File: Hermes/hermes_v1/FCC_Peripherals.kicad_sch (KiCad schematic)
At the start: 26 parts, among them J2 Connector_USB_B_Micro, J3 Conn_01x07, J4 Conn_02x07_Odd_Even, J5 Additional IO, J6 Micro_SD_Card, J7 IO Power, U5 MPU-6050, U6 MPL3115A2, U7 USBLC6-2P6

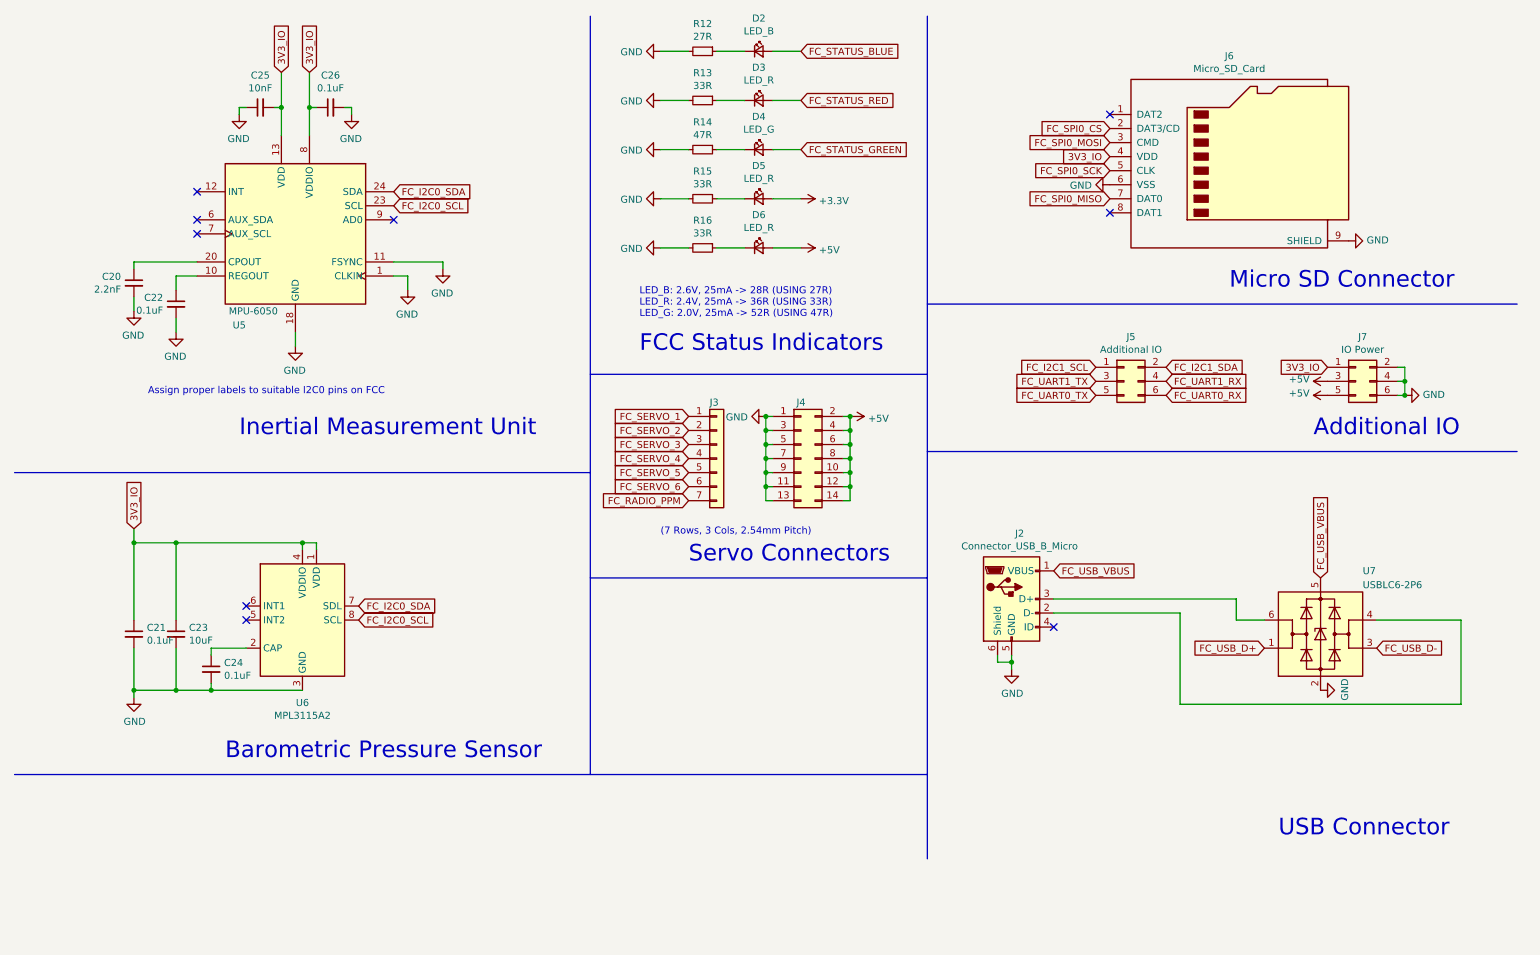
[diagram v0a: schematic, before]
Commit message: Hermes v2
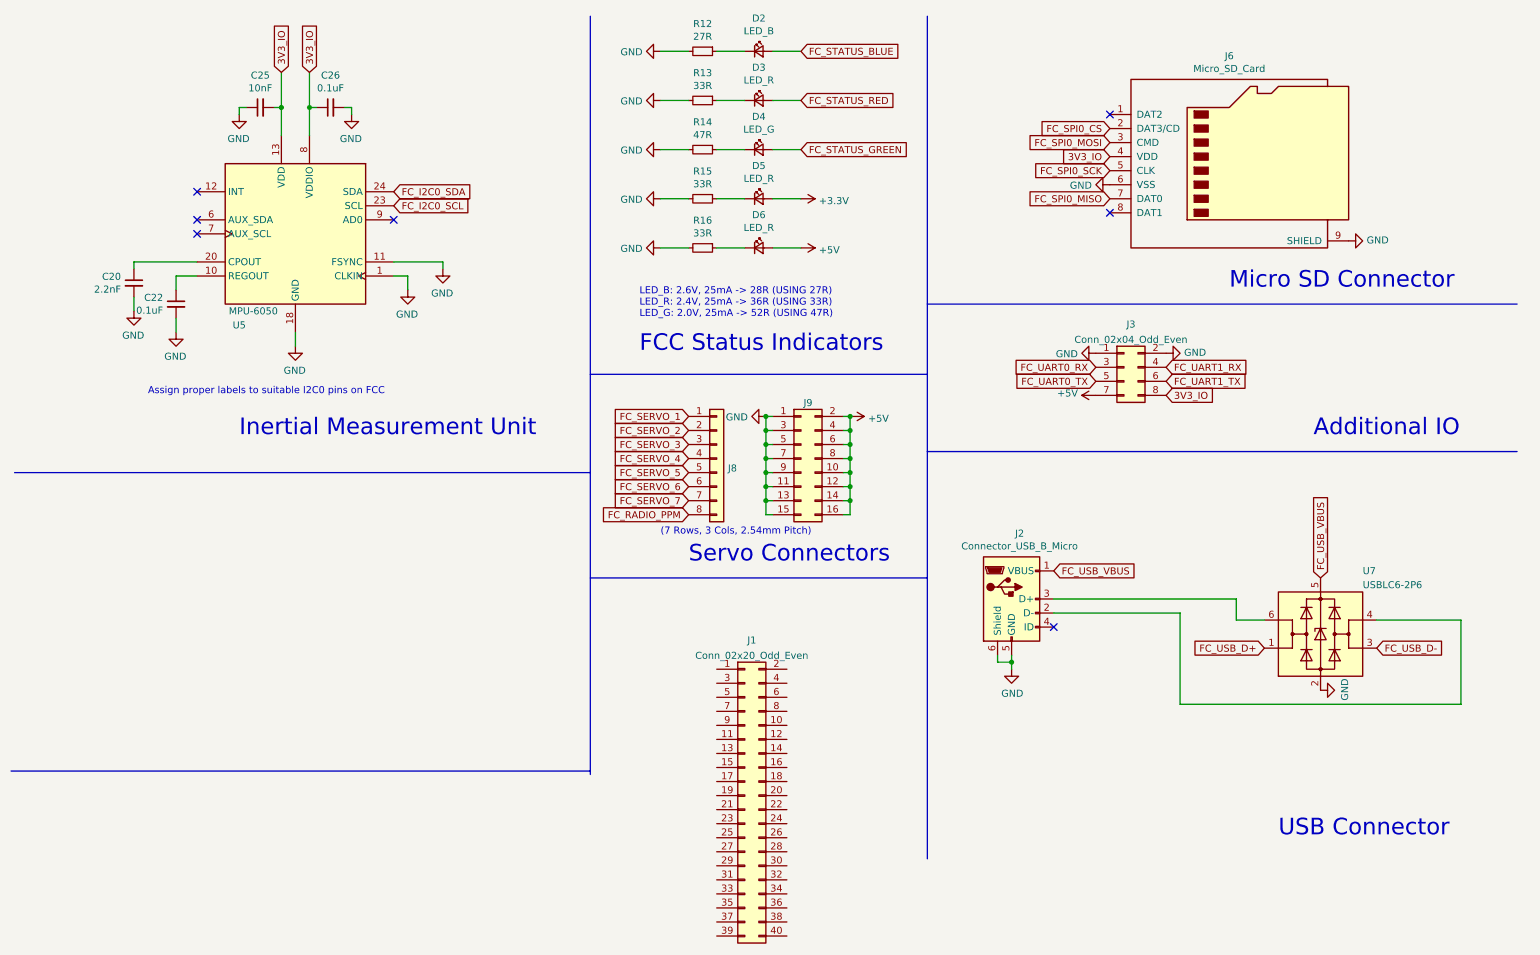
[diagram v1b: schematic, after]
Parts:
- removed C21, C24: 0.1uF, Capacitor_SMD:C_0402_1005Metric_Pad0.74x0.62mm_HandSolder, symbol Device:C_Small
- removed C23: 10uF, Capacitor_SMD:C_0402_1005Metric_Pad0.74x0.62mm_HandSolder, symbol Device:C_Small
- removed J3: Conn_01x07, Connector_PinHeader_2.54mm:PinHeader_1x07_P2.54mm_Vertical, symbol Connector_Generic:Conn_01x07
- removed J4: Conn_02x07_Odd_Even, Connector_PinHeader_2.54mm:PinHeader_2x07_P2.54mm_Vertical, symbol Connector_Generic:Conn_02x07_Odd_Even
- removed J5: Additional IO, Connector_PinHeader_2.54mm:PinHeader_2x03_P2.54mm_Vertical, symbol Connector_Generic:Conn_02x03_Odd_Even
- removed J7: IO Power, Connector_PinHeader_2.54mm:PinHeader_2x03_P2.54mm_Vertical, symbol Connector_Generic:Conn_02x03_Odd_Even
- removed U6: MPL3115A2, Package_LGA:NXP_LGA-8_3x5mm_P1.25mm_H1.1mm, symbol Sensor_Pressure:MPL3115A2
- added J1: Conn_02x20_Odd_Even, Connector_PinSocket_2.54mm:PinSocket_2x20_P2.54mm_Vertical, symbol Connector_Generic:Conn_02x20_Odd_Even
- added J3: Conn_02x04_Odd_Even, Connector_PinHeader_2.54mm:PinHeader_2x04_P2.54mm_Vertical, symbol Connector_Generic:Conn_02x04_Odd_Even
- added J8: Conn_01x08, Connector_PinHeader_2.54mm:PinHeader_1x08_P2.54mm_Vertical, symbol Connector_Generic:Conn_01x08
- added J9: Conn_02x08_Odd_Even, Connector_PinHeader_2.54mm:PinHeader_2x08_P2.54mm_Vertical, symbol Connector_Generic:Conn_02x08_Odd_Even
- J2: footprint Connector_USB:USB_Micro-B_Wuerth_614105150721_Vertical -> Connector_USB:USB_Micro-B_Amphenol_10118194_Horizontal
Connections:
- net +5V: now also J3.7 (Pin_7), J9.10 (Pin_10), J9.12 (Pin_12), J9.14 (Pin_14), J9.16 (Pin_16), J9.2 (Pin_2), J9.4 (Pin_4), J9.6 (Pin_6), J9.8 (Pin_8)
- net 3V3_IO: now also J3.8 (Pin_8)
- net FC_RADIO_PPM: now also J8.8 (Pin_8)
- net FC_SERVO_1: now also J8.1 (Pin_1)
- net FC_SERVO_2: now also J8.2 (Pin_2)
- net FC_SERVO_3: now also J8.3 (Pin_3)
- net FC_SERVO_4: now also J8.4 (Pin_4)
- net FC_SERVO_5: now also J8.5 (Pin_5)
- net FC_SERVO_6: now also J8.6 (Pin_6)
- net FC_UART0_RX: now also J3.3 (Pin_3)
- net FC_UART0_TX: now also J3.5 (Pin_5)
- net FC_UART1_RX: now also J3.4 (Pin_4)
- net FC_UART1_TX: now also J3.6 (Pin_6)
- net GND: now also J3.1 (Pin_1), J3.2 (Pin_2), J9.1 (Pin_1), J9.11 (Pin_11), J9.13 (Pin_13), J9.15 (Pin_15), J9.3 (Pin_3), J9.5 (Pin_5), J9.7 (Pin_7), J9.9 (Pin_9)
- new net FC_SERVO_7: J8.7 (Pin_7)
- no-connect marks 9 -> 7
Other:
- note removed: "Barometric Pressure Sensor"
